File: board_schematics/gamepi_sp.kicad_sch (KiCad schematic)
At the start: 25 parts, among them SW1 Power switch, SW2 UP, SW3 DOWN, SW4 LEFT, SW5 RIGHT, SW6 A, SW7 B, SW8 START, SW9 SELECT

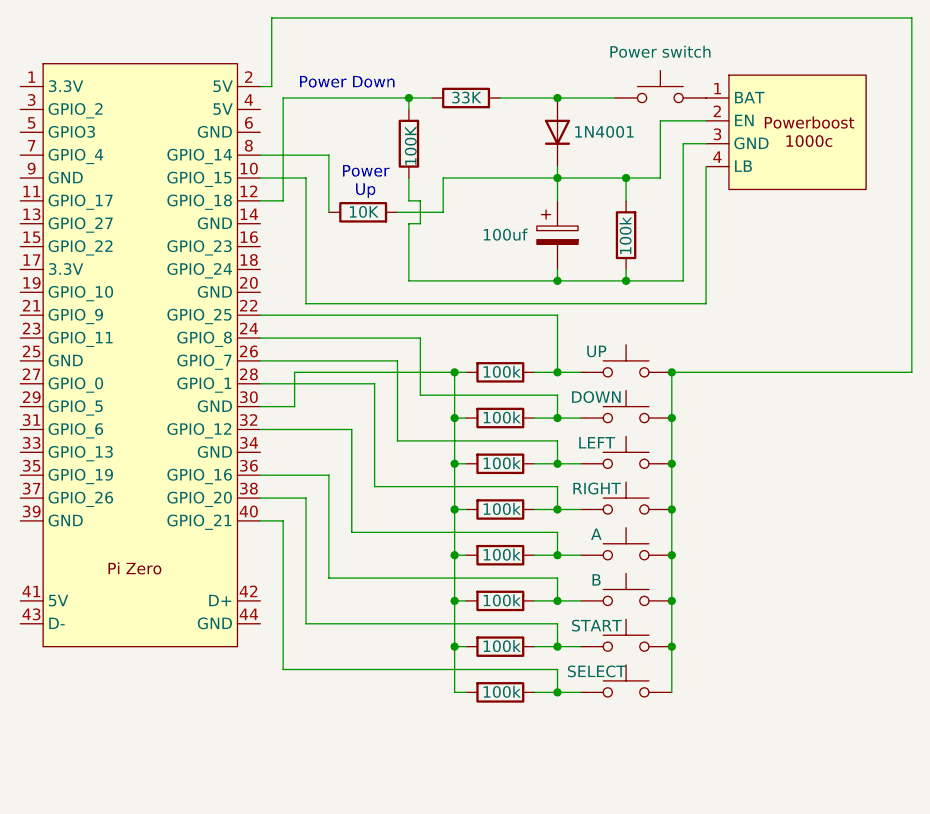
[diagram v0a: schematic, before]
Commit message: started documentation for assesment
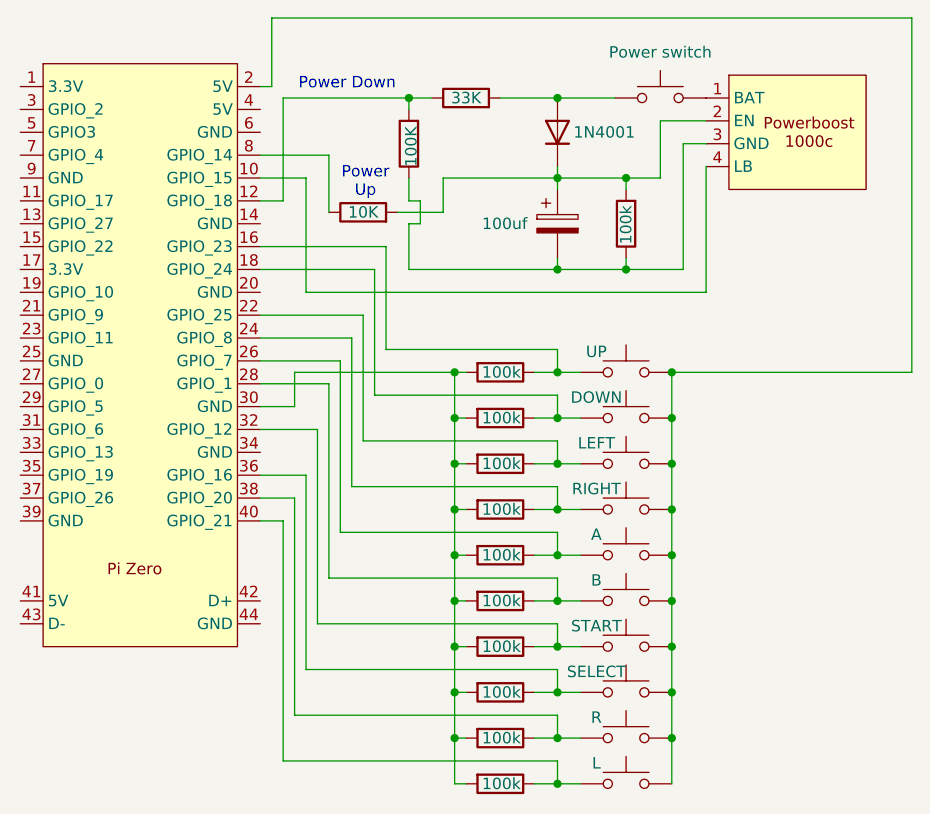
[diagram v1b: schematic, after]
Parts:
- added R13, R14: 100k, Resistor_SMD:R_0201_0603Metric, symbol Device:R
- added SW10: R, Button_Switch_THT:SW_PUSH_6mm, symbol Switch:SW_Push
- added SW11: L, Button_Switch_THT:SW_PUSH_6mm, symbol Switch:SW_Push
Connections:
- net at R5.1, SW5.1: now also U1.24 (GPIO_8); no longer U1.28 (GPIO_1)
- net at SW2.2, SW3.2, SW4.2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: now also SW10.2, SW11.2
- net at R6.1, SW4.1: now also U1.22 (GPIO_25); no longer U1.26 (GPIO_7)
- net at R7.1, SW3.1: now also U1.18 (GPIO_24); no longer U1.24 (GPIO_8)
- net at R8.1, SW9.1: now also U1.36 (GPIO_16); no longer U1.40 (GPIO_21)
- net at R10.2, R11.2, R12.2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: now also R13.2, R14.2
- net at R10.1, SW7.1: now also U1.28 (GPIO_1); no longer U1.36 (GPIO_16)
- net at R9.1, SW8.1: now also U1.32 (GPIO_12); no longer U1.38 (GPIO_20)
- net at R12.1, SW2.1: now also U1.16 (GPIO_23); no longer U1.22 (GPIO_25)
- net at R11.1, SW6.1: now also U1.26 (GPIO_7); no longer U1.32 (GPIO_12)
- new net: R13.1, SW10.1, U1.38 (GPIO_20)
- new net: R14.1, SW11.1, U1.40 (GPIO_21)
